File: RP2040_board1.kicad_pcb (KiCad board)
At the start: 2 copper layers, 90 x 60 mm, 191 parts, among them IC1 AP2112M-3.3TRG1, J1 Conn_01x02, J10 Conn_01x01, J11 Conn_01x01, J2 MEM2051-00-195-00-A, J3 Conn_01x03, J4 lefl_side, J5 right_side, J6 debug, J7 Conn_01x01, J8 Conn_01x02_Male, J9 USB_B_Mini, Q1 DMG9933USD-13, SW1 SW_SPST, SW2 SW_SPST, U1 W25Q128JVS, U2 RP2040, U3 APX810S05, U4 DHT11, U5 D1213A-02SM, U6 MCP79412, U7 DIO6012BCST6, Y1 ABLS-12.000MHZ-B4-T, Y2 32.7680kHz

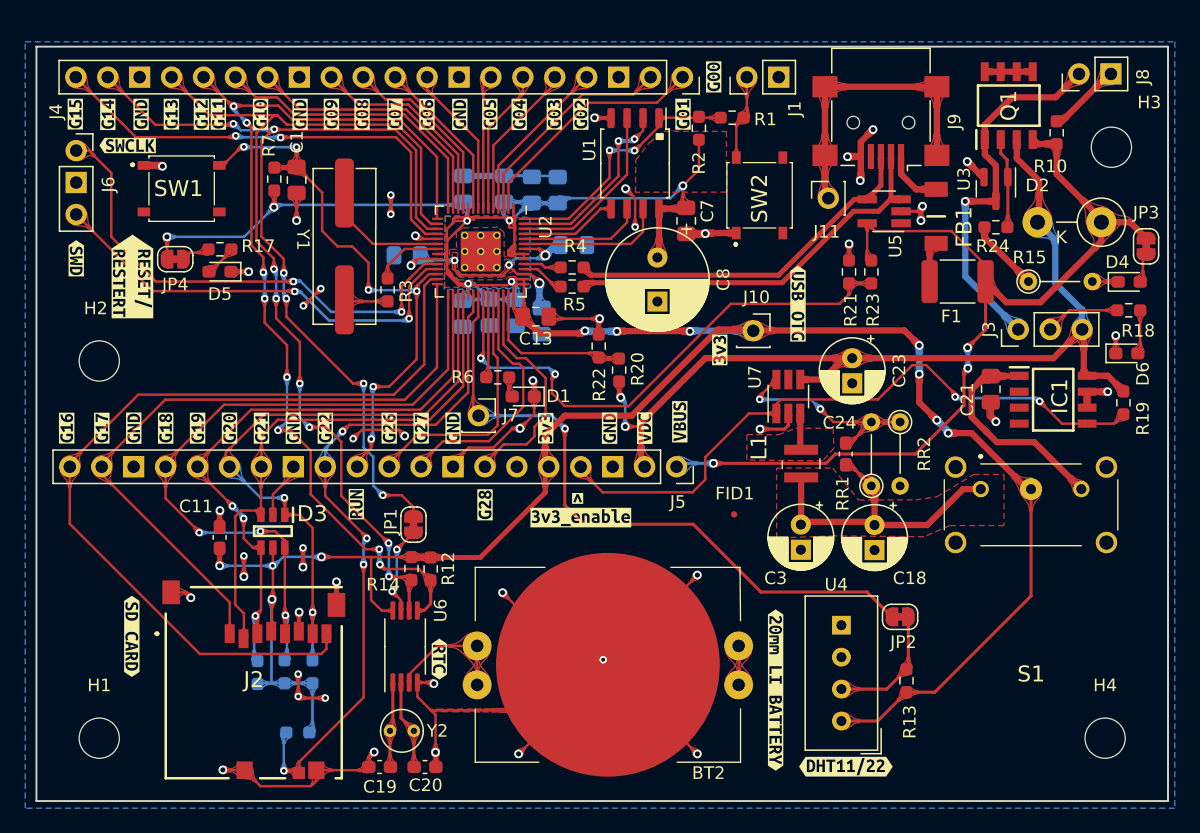
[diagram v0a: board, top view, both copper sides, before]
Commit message: f
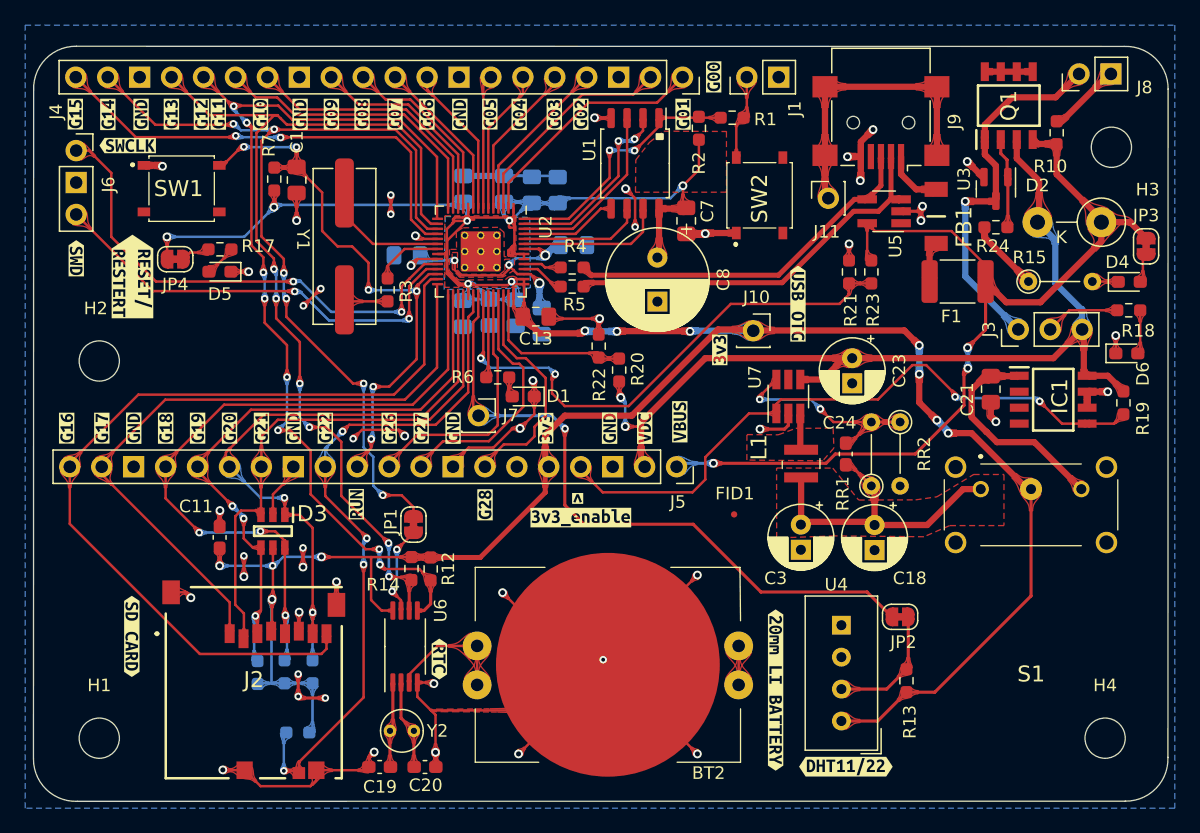
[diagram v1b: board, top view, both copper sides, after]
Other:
- board size 90 x 60 mm -> 90.2 x 60.1 mm
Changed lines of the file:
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@@
     (property "Sheetname" "Power")
     (attr through_hole)
-    (fp_text reference "J8" (at -0.23284 5.08616 90) (layer "F.SilkS")
+    (fp_text reference "J8" (at -1.07104 5.207 180) (layer "F.SilkS")
       (effects (font (size 1 1) (thickness 0.15)))
     )
@@
     (property "Sheetname" "Power")
     (attr exclude_from_pos_files)
-    (fp_text reference "JP3" (at -2.682 0 180) (layer "F.SilkS")
+    (fp_text reference "JP3" (at -2.4534 0 180) (layer "F.SilkS")
       (effects (font (size 1 1) (thickness 0.15)))
     )
@@
     (property "Sheetname" "")
     (attr exclude_from_pos_files)
-    (fp_text reference "H3" (at 3.012 -3.564) (layer "F.SilkS")
+    (fp_text reference "H3" (at 2.885 3.3702) (layer "F.SilkS")
       (effects (font (size 1 1) (thickness 0.15)))
     )
@@
   (gr_line (start 127.254 76.327) (end 126.8095 76.835) (layer "B.SilkS") (width 0.15))
   (gr_rect (start 120.3198 61.9506) (end 120.8278 62.357) (layer "F.SilkS") (width 0.15) (fill solid))
-  (gr_rect (start 71 55) (end 161 115) (layer "Edge.Cuts") (width 0.15) (fill none))
-  (gr_rect (start 71 55) (end 161 115) (layer "Margin") (width 0.15) (fill none))
+  (gr_arc (start 160.994489 111.527352) (mid 160.0454 113.9952) (end 157.603564 115.009339) (layer "Edge.Cuts") (width 0.1))
+  (gr_line (start 157.526752 54.981711) (end 74.171436 54.967461) (layer "Edge.Cuts") (width 0.1))
+  (gr_arc (start 70.780511 58.449448) (mid 71.729601 55.981602) (end 74.171436 54.967461) (layer "Edge.Cuts") (width 0.1))
+  (gr_line (start 70.780511 58.449448) (end 70.766261 111.629564) (layer "Edge.Cuts") (width 0.1))
+  (gr_line (start 74.248248 115.020489) (end 157.603564 115.009339) (layer "Edge.Cuts") (width 0.1))
+  (gr_line (start 160.994489 111.527352) (end 161.008739 58.372636) (layer "Edge.Cuts") (width 0.1))
+  (gr_arc (start 74.248248 115.020489) (mid 71.780372 114.071417) (end 70.766261 111.629564) (layer "Edge.Cuts") (width 0.1))
+  (gr_arc (start 157.526752 54.981711) (mid 159.9946 55.9308) (end 161.008739 58.372636) (layer "Edge.Cuts") (width 0.1))
+  (gr_line (start 70.780332 58.449631) (end 70.766082 111.629747) (layer "Margin") (width 0.1))
+  (gr_arc (start 70.780332 58.449631) (mid 71.729603 55.981955) (end 74.171257 54.967644) (layer "Margin") (width 0.1))
+  (gr_arc (start 157.526935 54.98189) (mid 159.994604 55.931162) (end 161.008922 58.372815) (layer "Margin") (width 0.1))
+  (gr_line (start 74.248069 115.020672) (end 157.603747 115.009518) (layer "Margin") (width 0.1))
+  (gr_arc (start 160.994672 111.527531) (mid 160.0454 113.9952) (end 157.603747 115.009518) (layer "Margin") (width 0.1))
+  (gr_line (start 157.526935 54.98189) (end 74.171257 54.967644) (layer "Margin") (width 0.1))
+  (gr_arc (start 74.248069 115.020672) (mid 71.780403 114.071401) (end 70.766082 111.629747) (layer "Margin") (width 0.1))
+  (gr_line (start 160.994672 111.527531) (end 161.008922 58.372815) (layer "Margin") (width 0.1))
   (dimension (type aligned) (layer "F.Fab")
     (pts (xy 161 55) (xy 71 55))
@@
         (xy 161.544 115.57)
         (xy 70.104 115.57)
-        (xy 70.104 54.61)
-        (xy 161.544 54.61)
+        (xy 70.104 53.2892)
+        (xy 161.544 53.2892)
       )
     )
